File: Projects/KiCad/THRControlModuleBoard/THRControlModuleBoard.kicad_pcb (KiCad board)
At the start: 2 copper layers, 119.8 x 119.8 mm, 31 parts, among them IC1 LTC1480CN8#PBF, IC2 LTC1480CN8#PBF, J1 Conn_01x02_Socket, J2 Conn_01x02_Socket, J3 Screw_Terminal_01x02, J4 Conn_01x04_Socket, J5 Conn_01x04_Socket, Q1 Q_PMOS_GDS, Q2 Q_PMOS_GDS, Q3 Q_PMOS_GDS, U1 LTC4416EMS#PBF, U2 MAX31856MUD+T, U3 NUCLEO-F303K8

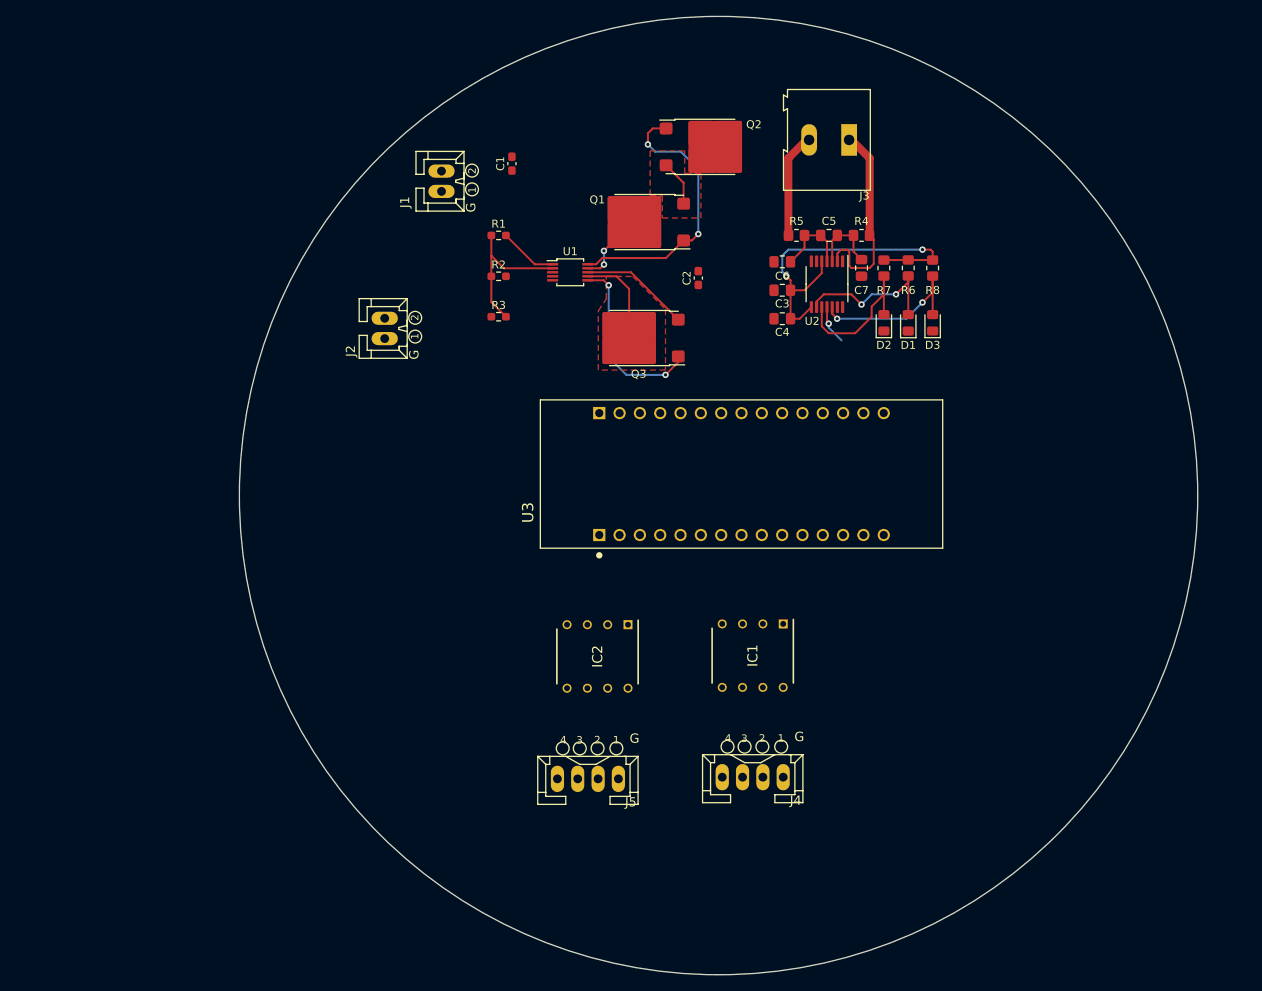
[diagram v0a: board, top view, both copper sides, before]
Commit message: THRControlModuleBoardの更新
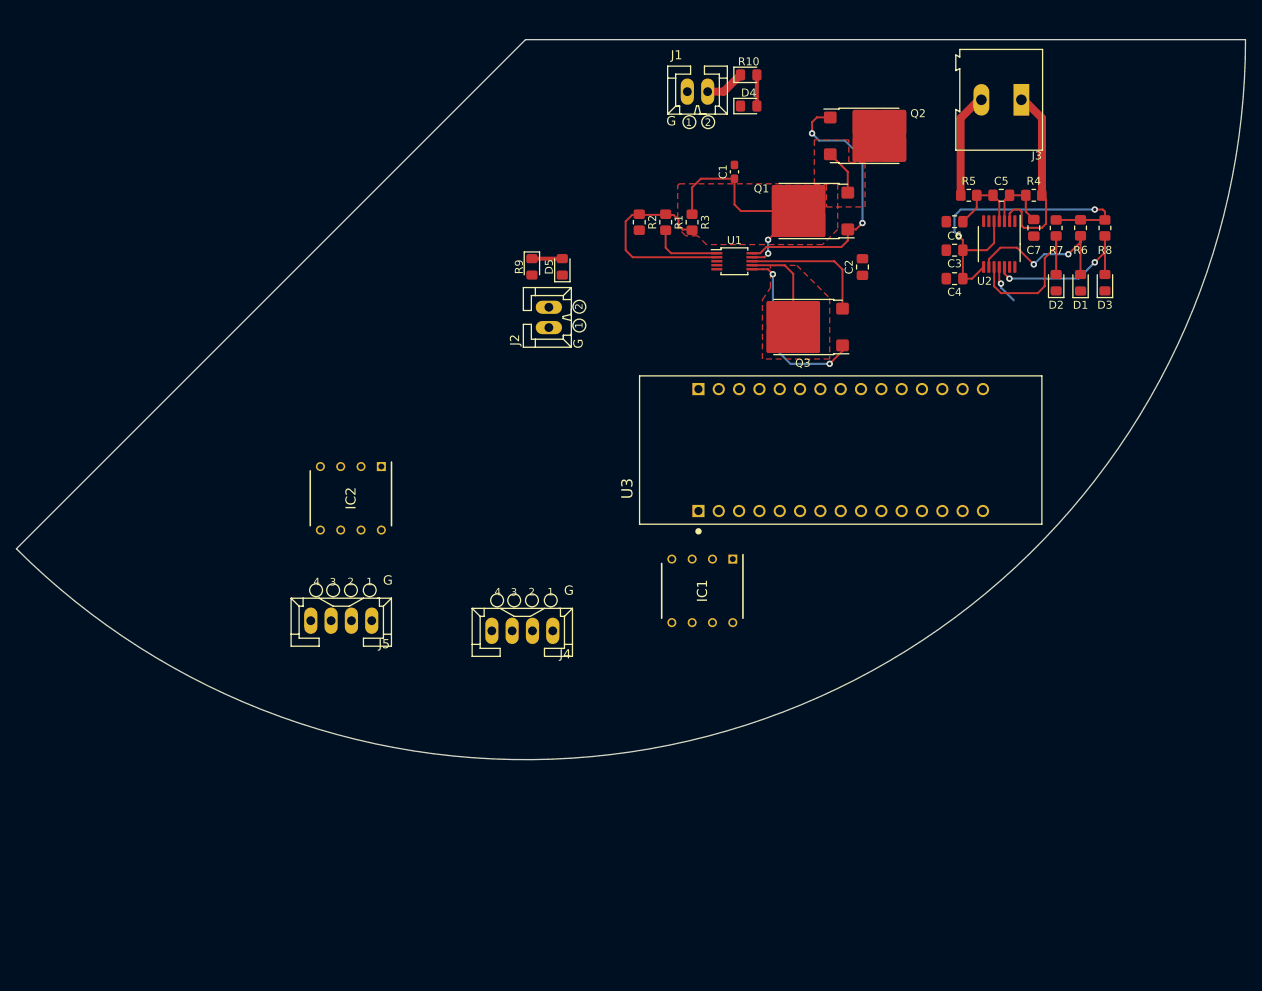
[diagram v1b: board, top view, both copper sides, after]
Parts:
- added D4: LED, LED_SMD:LED_0805_2012Metric_Pad1.15x1.40mm_HandSolder, F.Cu at (137.8, 40.6)
- added D5: LED, LED_SMD:LED_0805_2012Metric_Pad1.15x1.40mm_HandSolder, F.Cu at (114.5, 60.7)
- added R10: 1k, LED_SMD:LED_0805_2012Metric_Pad1.15x1.40mm_HandSolder, F.Cu at (137.8, 36.7)
- added R9: 1K, LED_SMD:LED_0805_2012Metric_Pad1.15x1.40mm_HandSolder, F.Cu at (110.7, 60.7)
- C2: footprint Capacitor_SMD:C_0603_1608Metric_Pad1.08x0.95mm_HandSolder -> Capacitor_SMD:C_0805_2012Metric_Pad1.18x1.45mm_HandSolder
- R1, R2, R3: footprint Resistor_SMD:R_0603_1608Metric_Pad0.98x0.95mm_HandSolder -> Resistor_SMD:R_0805_2012Metric_Pad1.20x1.40mm_HandSolder
- moved IC2 36.6 mm to (88.1, 89.6)
- moved J5 36.6 mm to (86.9, 104.9)
- moved J4 34.1 mm to (109.5, 106.2)
- moved J1 33.9 mm to (131.4, 38.8), turned to 0 degrees
- moved C1 27.8 mm to (136.0, 48.8)
- moved R3 26.9 mm to (130.7, 55.1), turned to -90 degrees
- moved C3 22.1 mm to (163.5, 58.6)
- moved C4 22.1 mm to (163.5, 62.2)
- moved C5 22.1 mm to (169.4, 51.8)
- moved C6 22.1 mm to (163.5, 55.1)
- moved D1 22.1 mm to (179.3, 62.7)
- moved D2 22.1 mm to (176.2, 62.7)
- moved D3 22.1 mm to (182.3, 62.7)
- moved R5 22.1 mm to (165.3, 51.8)
- moved R6 22.1 mm to (179.3, 55.8)
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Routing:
- net External Power Supply: track 8.22 -> 34.0 mm
- net Net-(U1-E1): track 19.3 -> 25.2 mm
- net Net-(D4-A): track 0.00 -> 3.90 mm
- net Net-(D5-A): track 0.00 -> 3.80 mm
- net Main Power Supply: track 13.8 -> 16.6 mm
- net Net-(U1-H1): track 7.39 -> 8.99 mm
- net Net-(D1-A): track 19.8 -> 20.7 mm
- net Net-(Q1-G): track 35.0 -> 35.8 mm
- net Net-(D2-A): track 20.4 -> 21.1 mm
- net +3.3V: track 44.2 -> 44.9 mm
- added copper zone on F.Cu, net External Power Supply
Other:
- board size 119.8 x 119.8 mm -> 153.6 x 90 mm
